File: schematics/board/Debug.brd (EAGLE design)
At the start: 84 x 54 mm, 29 parts, among them T1 2n7002, T2 2n7002

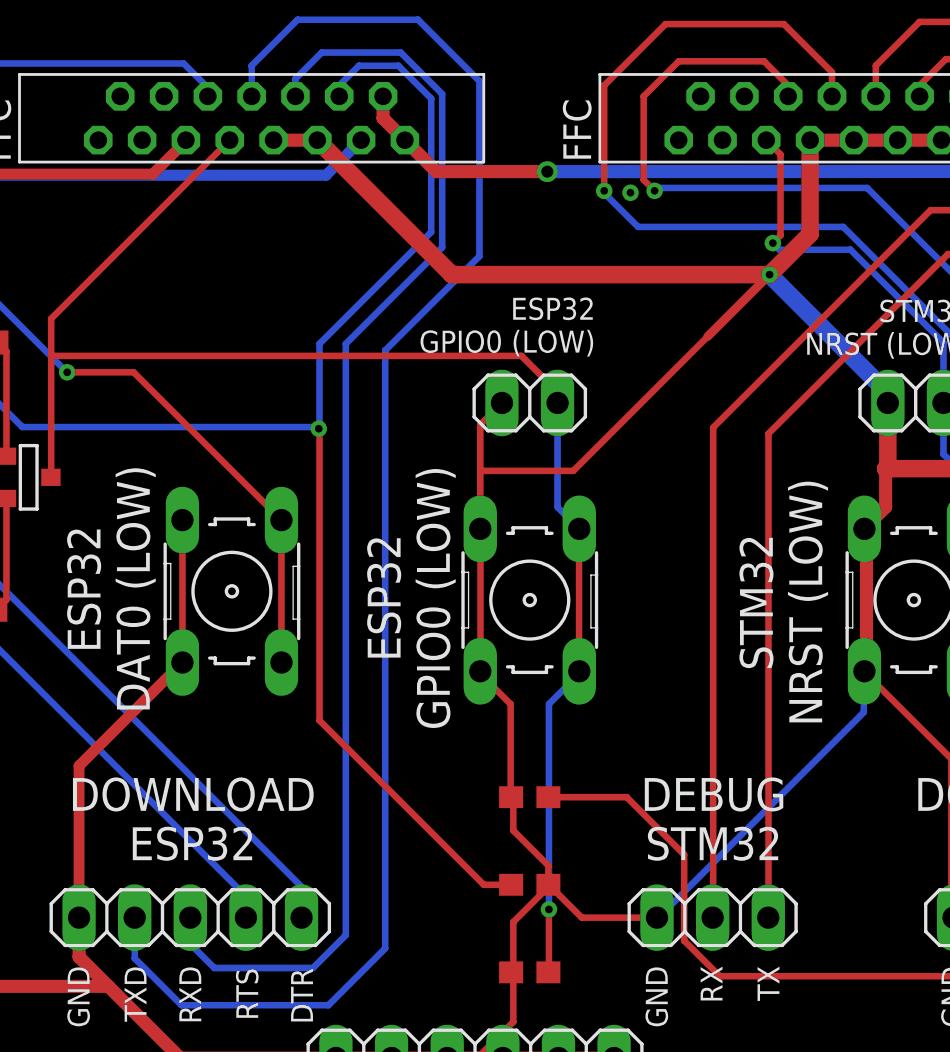
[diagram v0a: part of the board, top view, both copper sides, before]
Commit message: Исправлены герберы плат
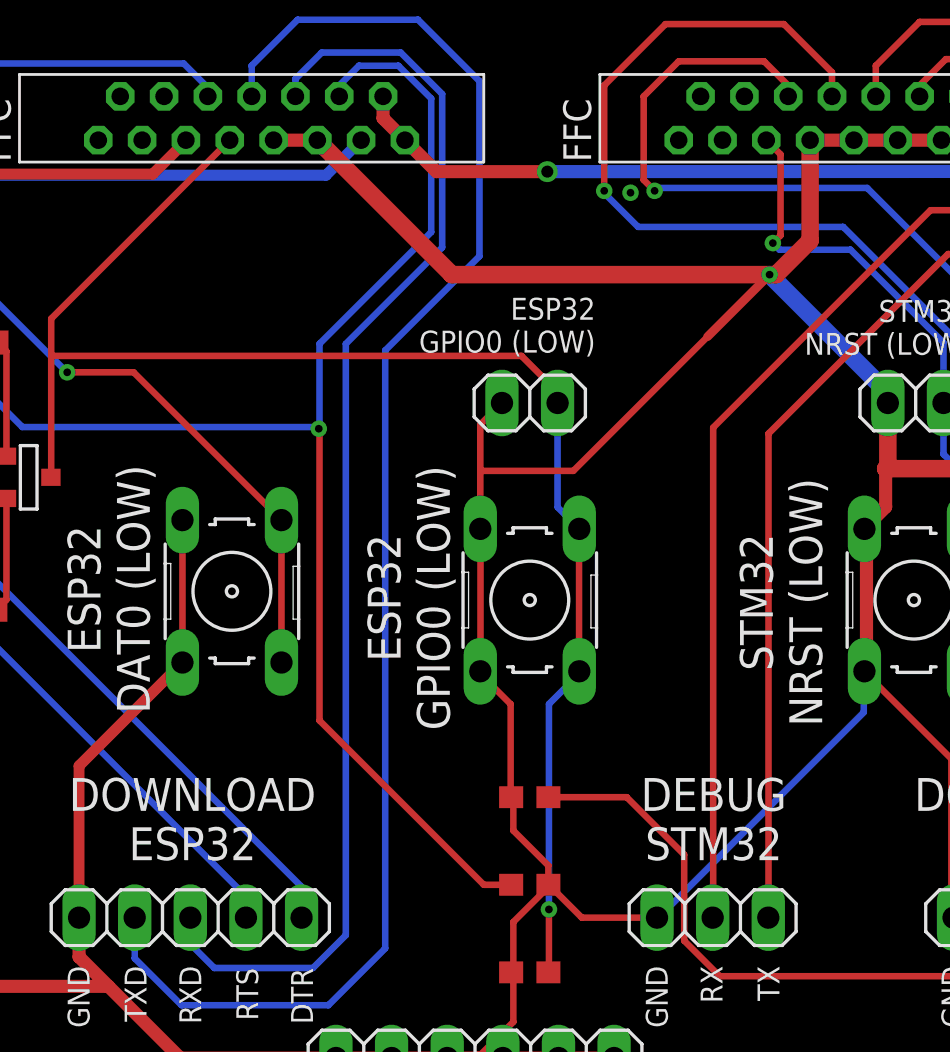
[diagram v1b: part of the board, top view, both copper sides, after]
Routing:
- net TX-E: track 71.5 -> 70.5 mm
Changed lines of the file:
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@@
 <contactref element="IO0" pad="4"/>
 <contactref element="C1" pad="2"/>
-<wire x1="42.75" y1="35" x2="42.77" y2="35" width="0.3" layer="16"/>
 <wire x1="42.375" y1="11.875" x2="42.375" y2="9" width="0.3" layer="1"/>
 <wire x1="42.375" y1="21.25" x2="42.375" y2="11.875" width="0.3" layer="16"/>
@@
 <wire x1="43.75" y1="29.25" x2="43.7606" y2="29.2512" width="0.3" layer="1"/>
 <wire x1="43.75" y1="22.75" x2="43.7606" y2="22.7488" width="0.3" layer="1"/>
-<wire x1="43.75" y1="29.375" x2="43.7606" y2="29.2512" width="0.3" layer="1"/>
 <via x="42.375" y="11.875" extent="1-16" drill="0.35"/>
 <contactref element="T2" pad="1"/>
@@
 <wire x1="7.86" y1="11.3" x2="5.95" y2="13.21" width="0.3" layer="16"/>
 <wire x1="25.6394" y1="29.6512" x2="25.6394" y2="23.1488" width="0.3" layer="1"/>
-<wire x1="54.3" y1="47" x2="54.3" y2="42.71" width="0.8" layer="1"/>
-<wire x1="54.3" y1="42.71" x2="52.45" y2="40.86" width="0.8" layer="1"/>
+<wire x1="54.3" y1="47" x2="54.3" y2="42.41" width="0.8" layer="1"/>
+<wire x1="54.3" y1="42.41" x2="52.75" y2="40.86" width="0.8" layer="1"/>
+<wire x1="52.75" y1="40.86" x2="52.45" y2="40.86" width="0.8" layer="1"/>
 <wire x1="52.45" y1="40.86" x2="49.615" y2="38.025" width="0.4" layer="1"/>
-<wire x1="40.23" y1="35" x2="40.23" y2="35.325" width="0.4" layer="1"/>
 <wire x1="25.6394" y1="23.1488" x2="20.92" y2="18.4294" width="0.5" layer="1"/>
 <wire x1="20.92" y1="18.4294" x2="20.92" y2="11.5" width="0.5" layer="1"/>
@@
 <wire x1="39.2" y1="49.7" x2="39.2" y2="41.7" width="0.3" layer="16"/>
 <contactref element="DOWNLOAD_ESP32" pad="2"/>
-<wire x1="23.46" y1="11.5" x2="23.46" y2="12.5" width="0.3" layer="1"/>
 <wire x1="34.9" y1="10.1" x2="32.3" y2="7.5" width="0.3" layer="16"/>
 <wire x1="32.3" y1="7.5" x2="25.6" y2="7.5" width="0.3" layer="16"/>
